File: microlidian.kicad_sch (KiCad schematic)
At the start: 31 parts, among them J1 Conn_02x05_Odd_Even, J11 Backboard Conn 1, J12 Frontboard Conn 1, J13 Backboard Conn 2, J14 Frontboard Conn 2, J2 ST7789 TFT socket, J3 Expansion header, J4 ADS1015 digital side, J5 ADS1015 analog side, J7 TRS MIDI Out, SW1 RotaryEncoder_Switch, SW2 Back button, U1 SeeeduinoXIAO, U2 L78L05_TO92

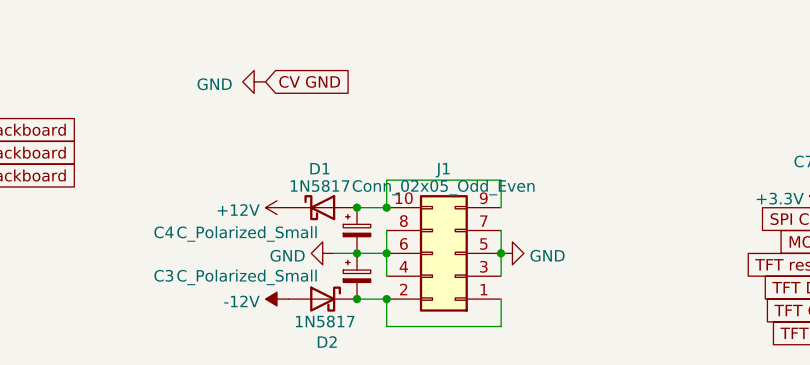
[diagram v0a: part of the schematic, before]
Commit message: some minor updates
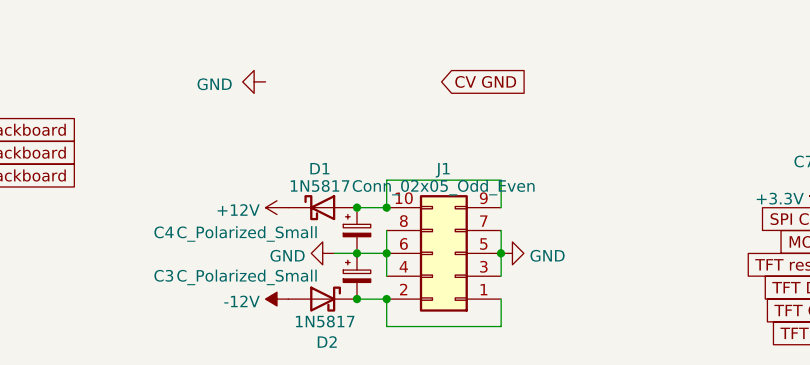
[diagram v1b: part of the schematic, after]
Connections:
- net GND: no longer J5.5 (Pin_5)
- new net CV GND: J5.5 (Pin_5)
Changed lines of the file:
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@@
     )
   )
-  (global_label "CV GND" (shape input) (at 180.848 20.32 0) (fields_autoplaced)
+  (global_label "CV GND" (shape input) (at 200.406 20.32 0) (fields_autoplaced)
     (effects (font (size 1.27 1.27)) (justify left))
-    (property "Intersheetrefs" "${INTERSHEET_REFS}" (at 190.0907 20.32 0)
+    (property "Intersheetrefs" "${INTERSHEET_REFS}" (at 209.6487 20.32 0)
       (effects (font (size 1.27 1.27)) (justify left) hide)
     )
